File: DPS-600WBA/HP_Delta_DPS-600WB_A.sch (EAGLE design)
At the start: 17 parts, among them Q1 20n60c3 TO-247

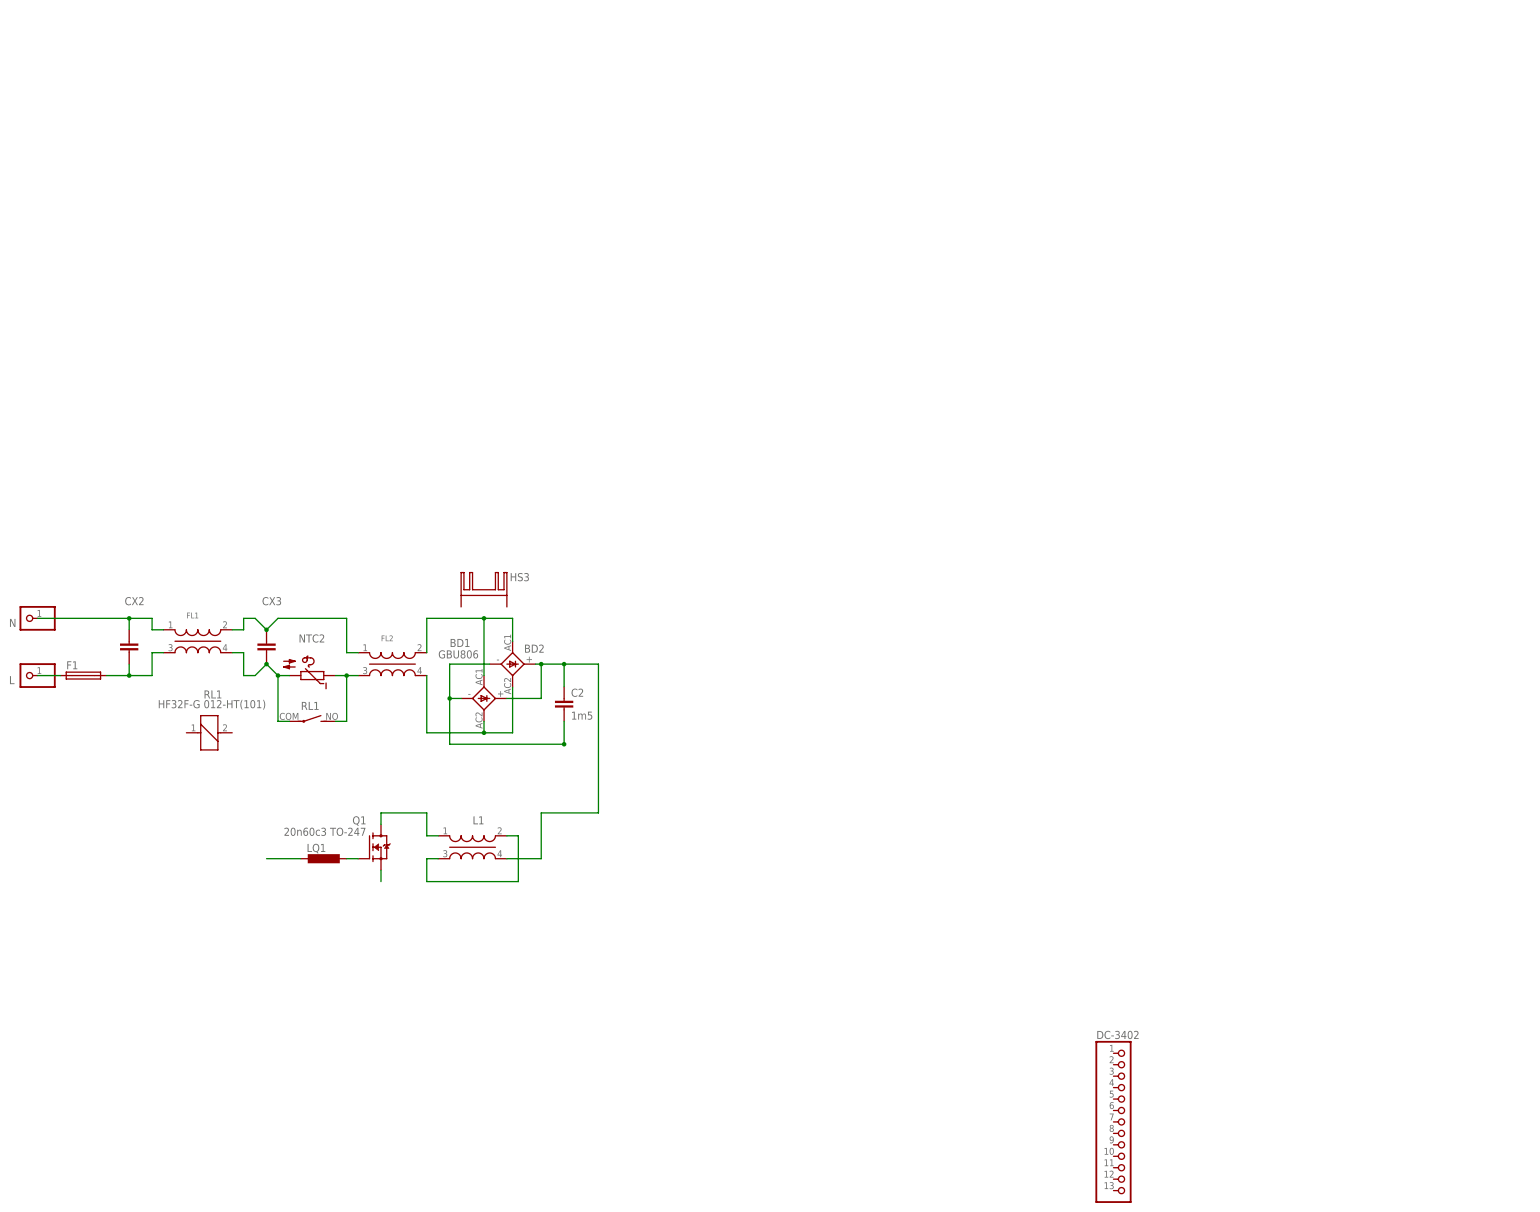
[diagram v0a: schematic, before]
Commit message: .
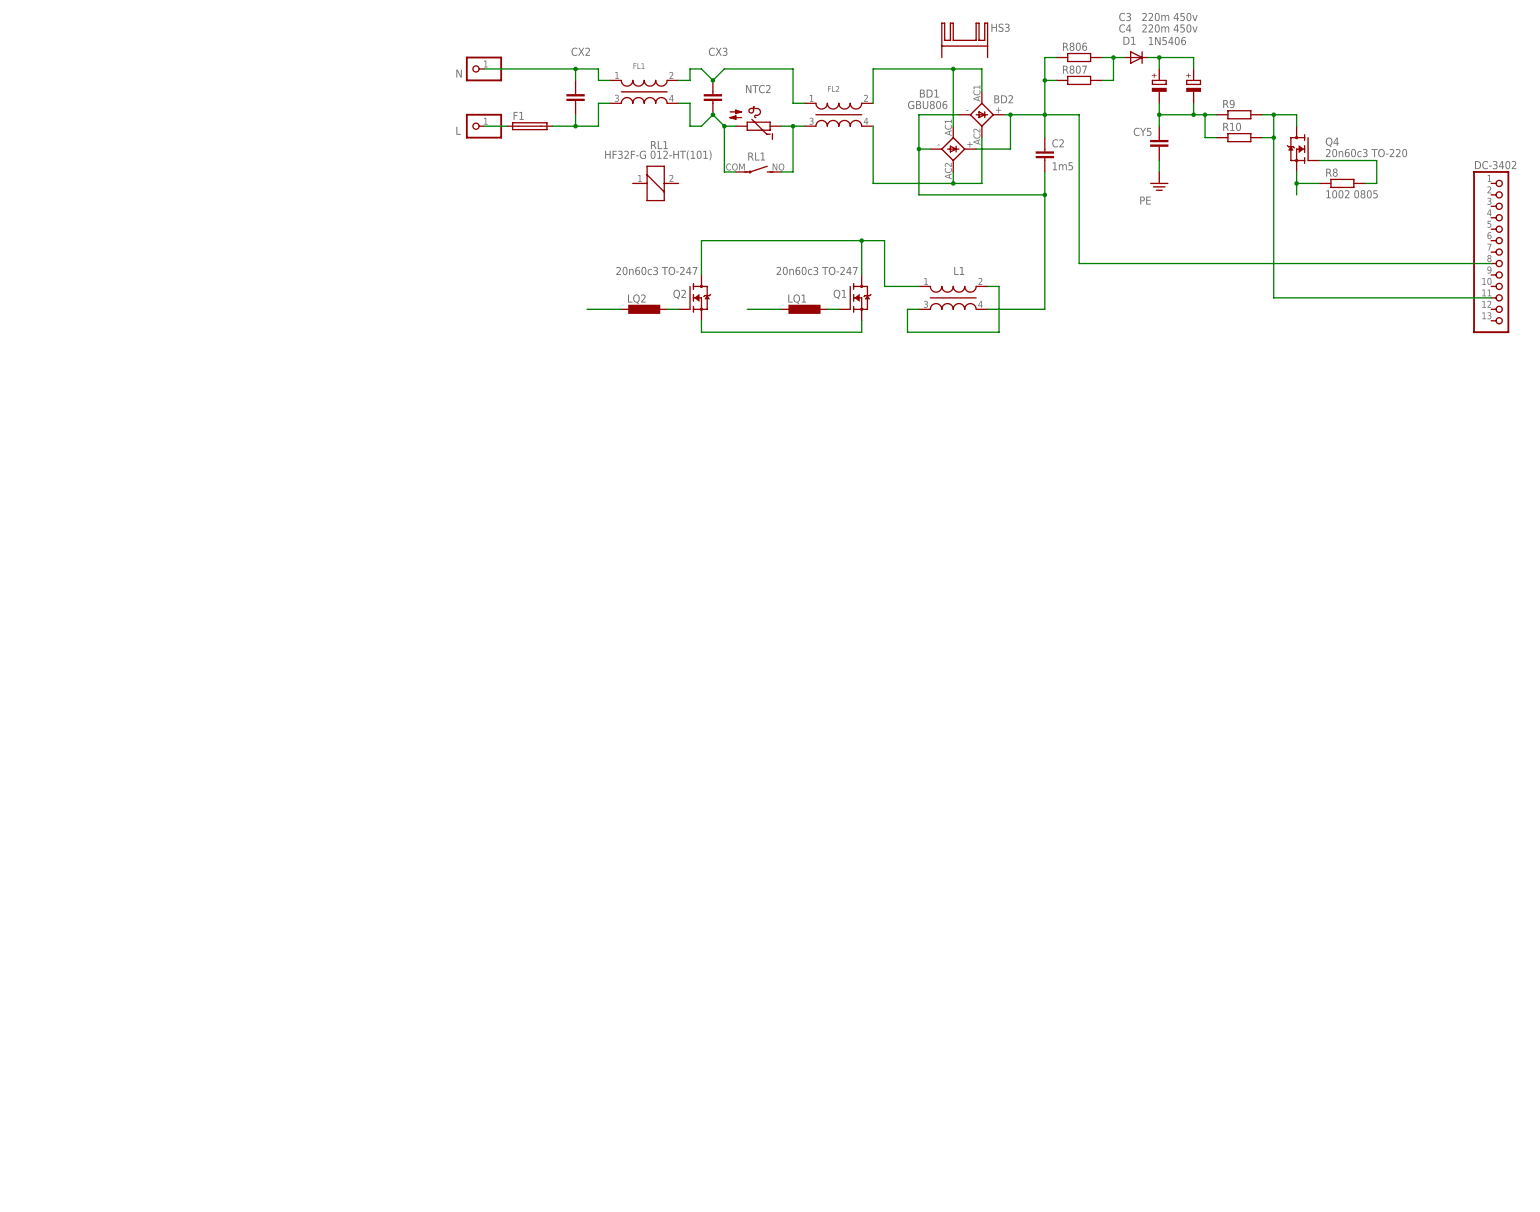
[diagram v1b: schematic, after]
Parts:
- added C3, C4: 220m 450v, rcl:CPOL-EUSANYO_E7
- added CY5: (no value), rcl:C-EU025-040X050
- added D1: 1N5406, diode:1N4942
- added LQ2: (no value), rcl:L-EU0204/5
- added Q2: 20n60c3 TO-247, transistor-fet:SPW47N60S5
- added Q4: 20n60c3 TO-220, transistor-fet:SPW47N60S5
- added R10, R9: (no value), rcl:R-EU_0204/7
- added R8: 1002 0805, rcl:R-EU_R0805
- added R806, R807: (no value), rcl:R-EU_0309/12
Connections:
- new net N$16: L1.1, Q1.D, Q2.D
- new net N$17: LQ2.1, Q2.G
- new net N$18: LQ2.2
- new net N$19: Q1.S, Q2.S
- new net N$20: C3.-, C4.-, CY5.1, R10.1, R9.1
- new net N$21: Q4.G, R8.2
- new net N$22: DC-3402.11, Q4.D, R10.2, R9.2
- new net N$23: Q4.S, R8.1
- new net PE: CY5.2
- net N$11: now also D1.A, R806.2, R807.2; no longer L1.1, Q1.D
- net N$13: now also DC-3402.8, R806.1, R807.1; no longer L1.4
- net N$15: now also C3.+, C4.+, D1.C; no longer Q1.S
- net N$3: now also L1.4
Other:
- moved on the sheet: BD1, BD2, C2, CX2, CX3, DC-3402, F1, FL1, FL2, HS3, L, L1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
